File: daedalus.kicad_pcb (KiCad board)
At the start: 4 copper layers, 130.1 x 55.1 mm, 98 parts, among them J1 CAN Bus, J2 CAN Bus, J5 A Terminal, J6 B Terminal, J7 C Terminal, J9 USB_B_Micro, Q1 AO3401A, U1 XT30, U10 TPH, U11 TPH, U12 TPH, U13 TPH, U14 USBLC6-2SC6, U2 XT30, U3 MP2359DJ-LF-Z, U5 DRV8323RH, U6 MCP2542, U7 STM32F405RGTx, U8 TPH, U9 TPH, Y1 16MHz

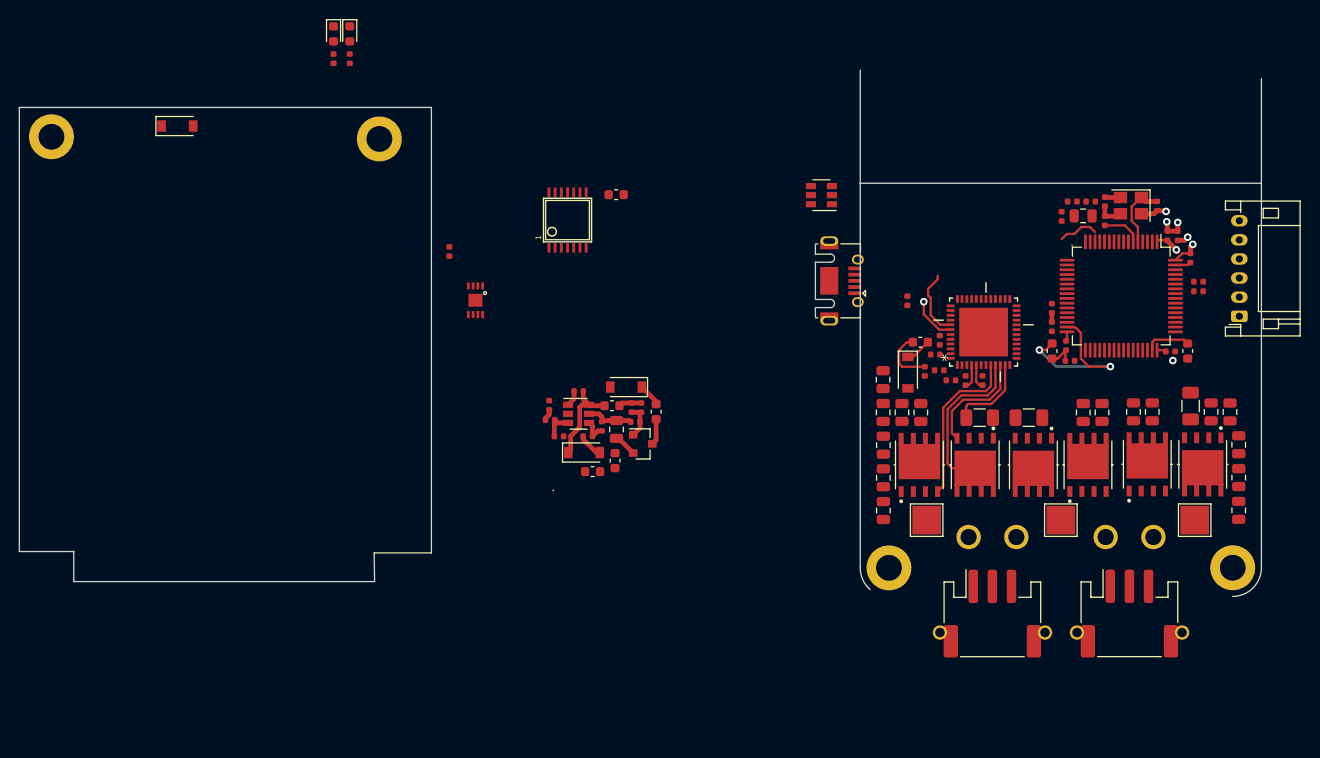
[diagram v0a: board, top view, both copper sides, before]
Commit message: Finished rough layout v3
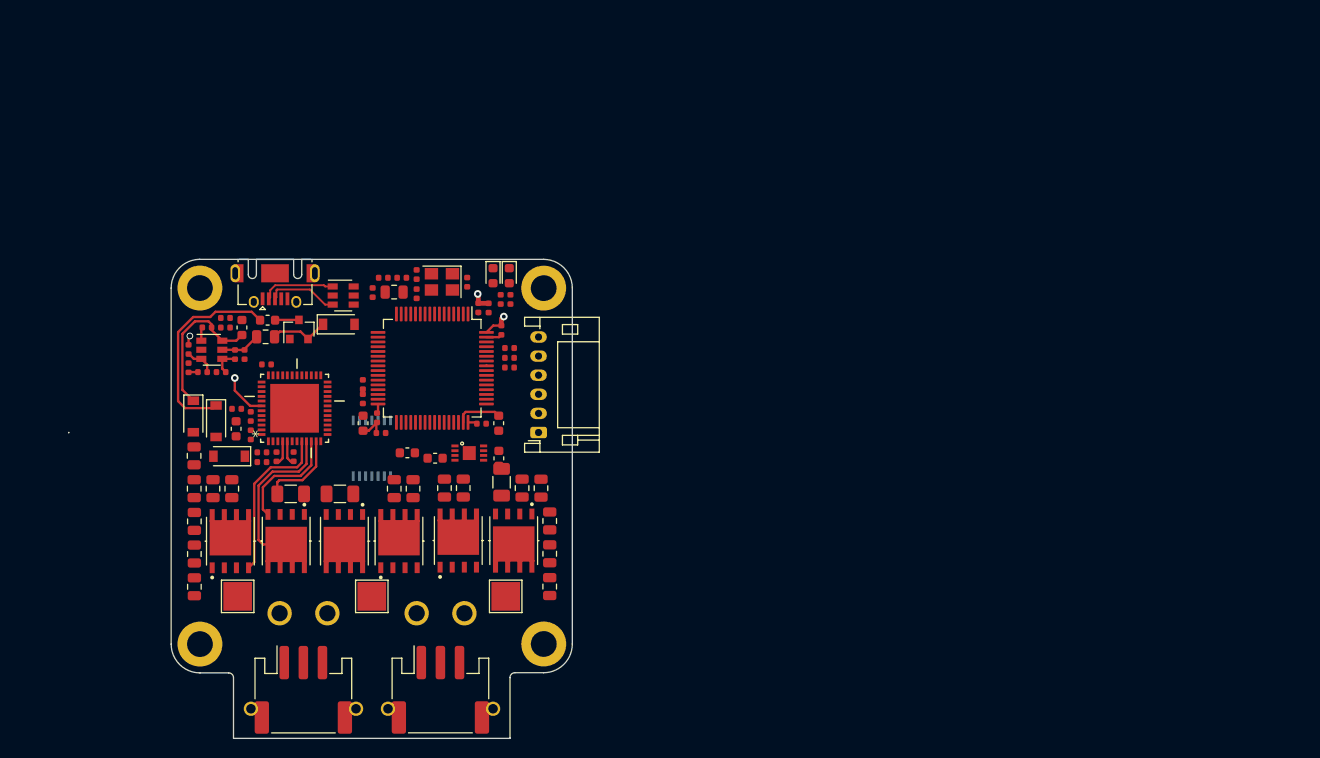
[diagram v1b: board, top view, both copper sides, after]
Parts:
- 1: moved to B.Cu
- moved SWD1 74.4 mm to (161.4, 93.5)
- moved C25 72.7 mm to (153.9, 77.8)
- moved R14 72.7 mm to (132.5, 96.6), turned to 180 degrees
- moved C16 72.6 mm to (134.0, 96.1)
- moved C21 72.6 mm to (135.8, 96.1)
- moved C28 72.6 mm to (151.6, 99.4)
- moved C29 72.6 mm to (161.7, 99.4)
- moved C31 72.6 mm to (162.6, 109.7)
- moved C32 72.6 mm to (159.7, 99.4)
- moved C34 72.6 mm to (153.5, 99.4)
- moved C35 72.6 mm to (129.3, 99.4)
- moved C38 72.6 mm to (162.6, 106.2)
- moved C39 72.6 mm to (125.4, 109.7)
- moved C41 72.6 mm to (162.6, 102.8)
- moved C42 72.6 mm to (125.4, 99.4)
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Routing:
- net Net-(D1-Pad1): track 2.41 -> 21.4 mm
- net Net-(C19-Pad2): track 17.6 -> 0.00 mm, vias 2 -> 0
- net BGND: track 18.4 -> 6.73 mm, vias 4 -> 1
- net PWM_C: track 11.4 -> 0.00 mm
- net USB_CONN_D-: track 0.00 -> 7.77 mm
- net USB_CONN_D+: track 0.00 -> 7.54 mm
- net HSE_IN: track 7.17 -> 0.00 mm
- net VDD: track 12.0 -> 5.93 mm, vias 3 -> 2
- net BUCK_SW: track 9.65 -> 15.7 mm
- net +5VD: track 6.03 -> 0.00 mm
- net HSE_OUT: track 4.17 -> 0.00 mm
- net Net-(D2-Pad1): track 2.38 -> 6.26 mm
- net Net-(C26-Pad2): track 2.77 -> 0.00 mm
- net SW: track 2.73 -> 0.00 mm
- net Net-(C2-Pad1): track 5.10 -> 4.23 mm
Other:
- board size 130.1 x 55.1 mm -> 52.8 x 50.2 mm
